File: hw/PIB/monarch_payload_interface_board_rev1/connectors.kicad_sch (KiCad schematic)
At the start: 15 parts, among them J1 5037630291, J10 5037630491, J11 5037630691, J12 5037630691, J13 5037630491, J14 5037630491, J15 5037630691, J2 5037630291, J3 5037630691, J4 5037630691, J5 5037630691, J6 5037630691, J7 5037630691, J8 5037630691, J9 5037630491

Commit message: minor tweaks
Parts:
- J15: footprint CONN_5037630000-SD_06_MOL -> 5037630691:CONN_5037630000-SD_06_MOL
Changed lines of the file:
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@@
 			)
 		)
-		(property "Footprint" "CONN_5037630000-SD_06_MOL"
+		(property "Footprint" "5037630691:CONN_5037630000-SD_06_MOL"
 			(at 171.45 109.22 0)
 			(effects

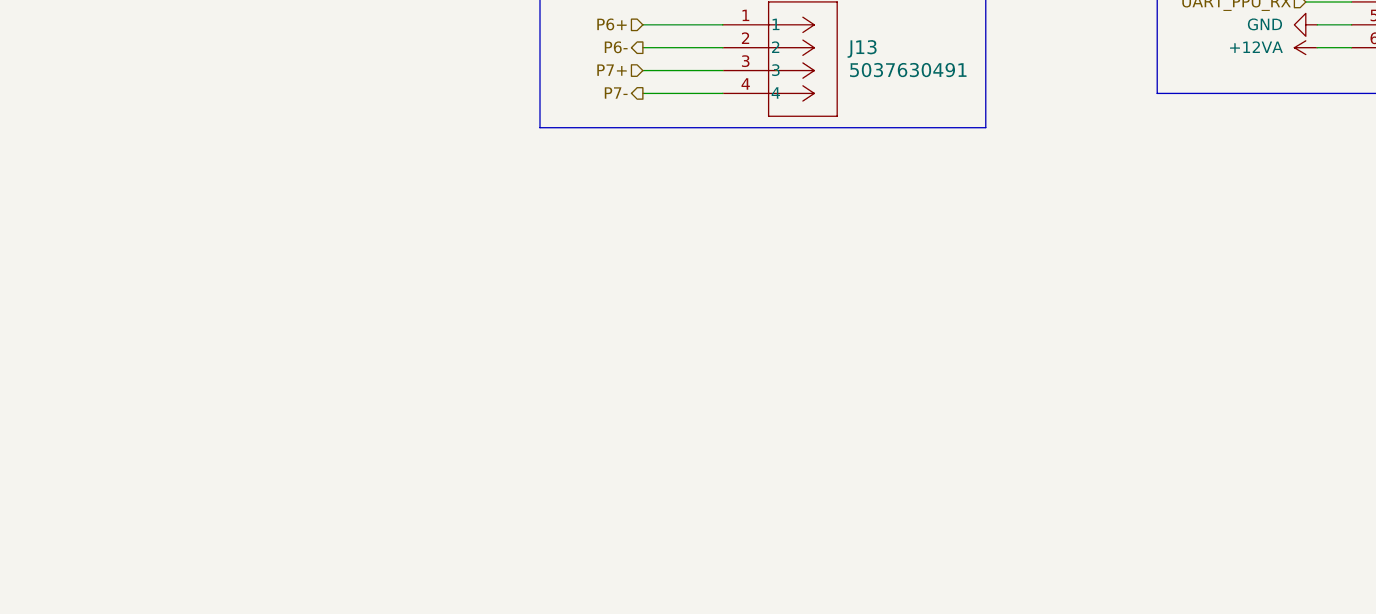
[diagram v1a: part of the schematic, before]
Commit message: BOOT PIN FIX + NRST PIN FIX
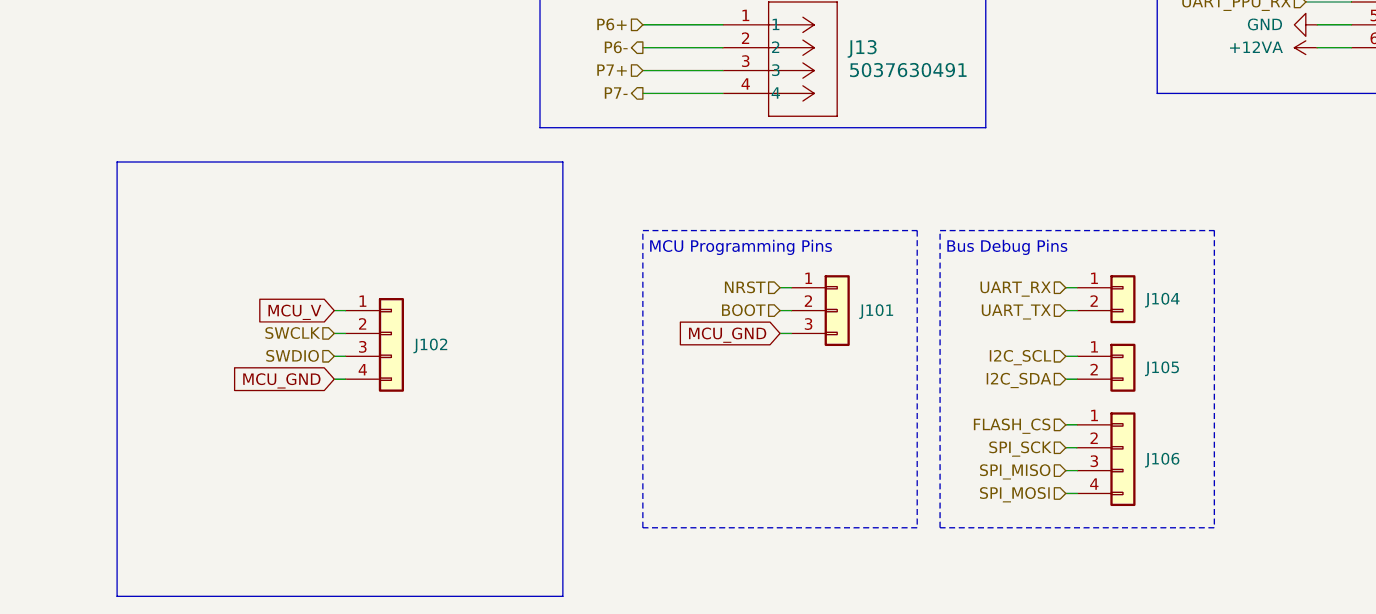
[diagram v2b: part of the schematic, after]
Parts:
- added J101: Conn_01x03, Connector_PinHeader_1.27mm:PinHeader_1x03_P1.27mm_Vertical, symbol Connector_Generic:Conn_01x03
- added J102: Conn_01x04, Connector_PinHeader_2.54mm:PinHeader_1x04_P2.54mm_Vertical, symbol Connector_Generic:Conn_01x04
- added J104: Conn_01x02, Connector_PinHeader_2.54mm:PinHeader_1x02_P2.54mm_Vertical, symbol Connector_Generic:Conn_01x02
- added J105: Conn_01x02, Connector_PinHeader_1.27mm:PinHeader_1x02_P1.27mm_Vertical, symbol Connector_Generic:Conn_01x02
- added J106: Conn_01x04, Connector_PinHeader_1.27mm:PinHeader_1x04_P1.27mm_Vertical, symbol Connector_Generic:Conn_01x04
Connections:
- new net BOOT: J101.2 (Pin_2)
- new net FLASH_CS: J106.1 (Pin_1)
- new net I2C_SCL: J105.1 (Pin_1)
- new net I2C_SDA: J105.2 (Pin_2)
- new net MCU_GND: J101.3 (Pin_3), J102.4 (Pin_4)
- new net MCU_V: J102.1 (Pin_1)
- new net NRST: J101.1 (Pin_1)
- new net SPI_MISO: J106.3 (Pin_3)
- new net SPI_MOSI: J106.4 (Pin_4)
- new net SPI_SCK: J106.2 (Pin_2)
- new net SWCLK: J102.2 (Pin_2)
- new net SWDIO: J102.3 (Pin_3)
- new net UART_RX: J104.1 (Pin_1)
- new net UART_TX: J104.2 (Pin_2)
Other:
- note added: "Bus Debug Pins"
- note added: "MCU Programming Pins"

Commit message: New REV2 addition
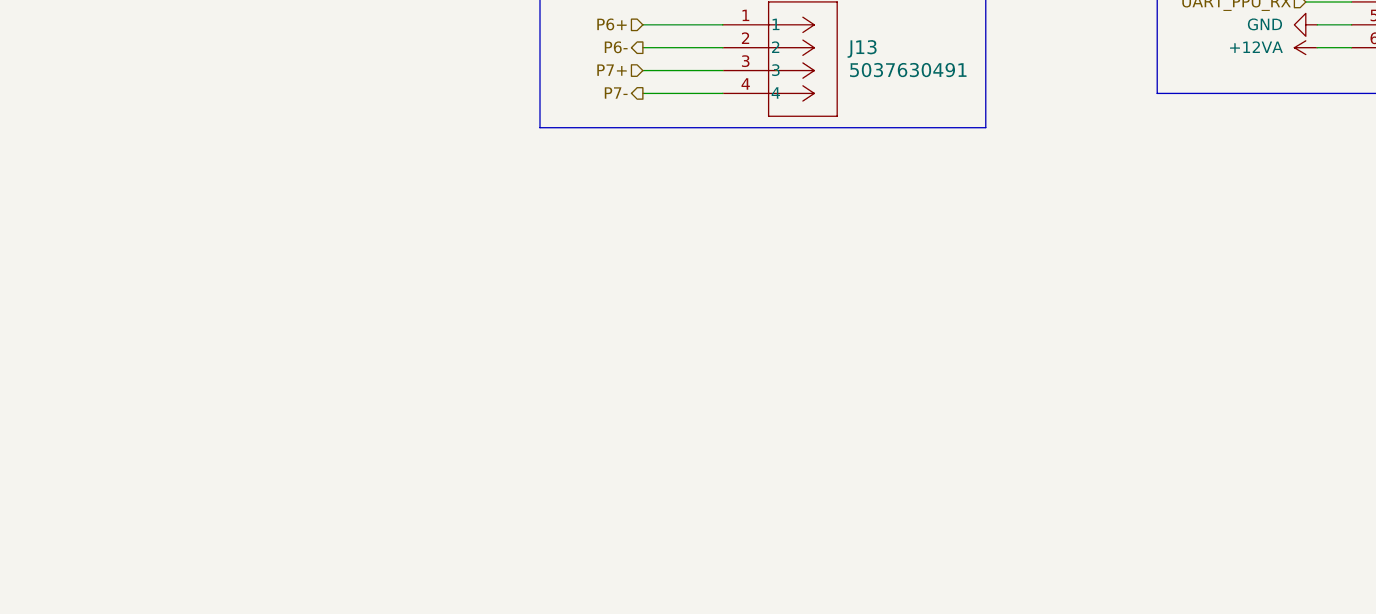
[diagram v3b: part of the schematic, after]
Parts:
- removed J101: Conn_01x03, Connector_PinHeader_1.27mm:PinHeader_1x03_P1.27mm_Vertical, symbol Connector_Generic:Conn_01x03
- removed J102: Conn_01x04, Connector_PinHeader_2.54mm:PinHeader_1x04_P2.54mm_Vertical, symbol Connector_Generic:Conn_01x04
- removed J104: Conn_01x02, Connector_PinHeader_2.54mm:PinHeader_1x02_P2.54mm_Vertical, symbol Connector_Generic:Conn_01x02
- removed J105: Conn_01x02, Connector_PinHeader_1.27mm:PinHeader_1x02_P1.27mm_Vertical, symbol Connector_Generic:Conn_01x02
- removed J106: Conn_01x04, Connector_PinHeader_1.27mm:PinHeader_1x04_P1.27mm_Vertical, symbol Connector_Generic:Conn_01x04
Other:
- note removed: "Bus Debug Pins"
- note removed: "MCU Programming Pins"
